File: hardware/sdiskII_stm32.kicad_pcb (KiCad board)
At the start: 2 copper layers, 67 x 55.5 mm, 8 parts, among them J2 APPLE_SDISKII, U2 MicroSD_SDIO, U8 DM-OLED096-636

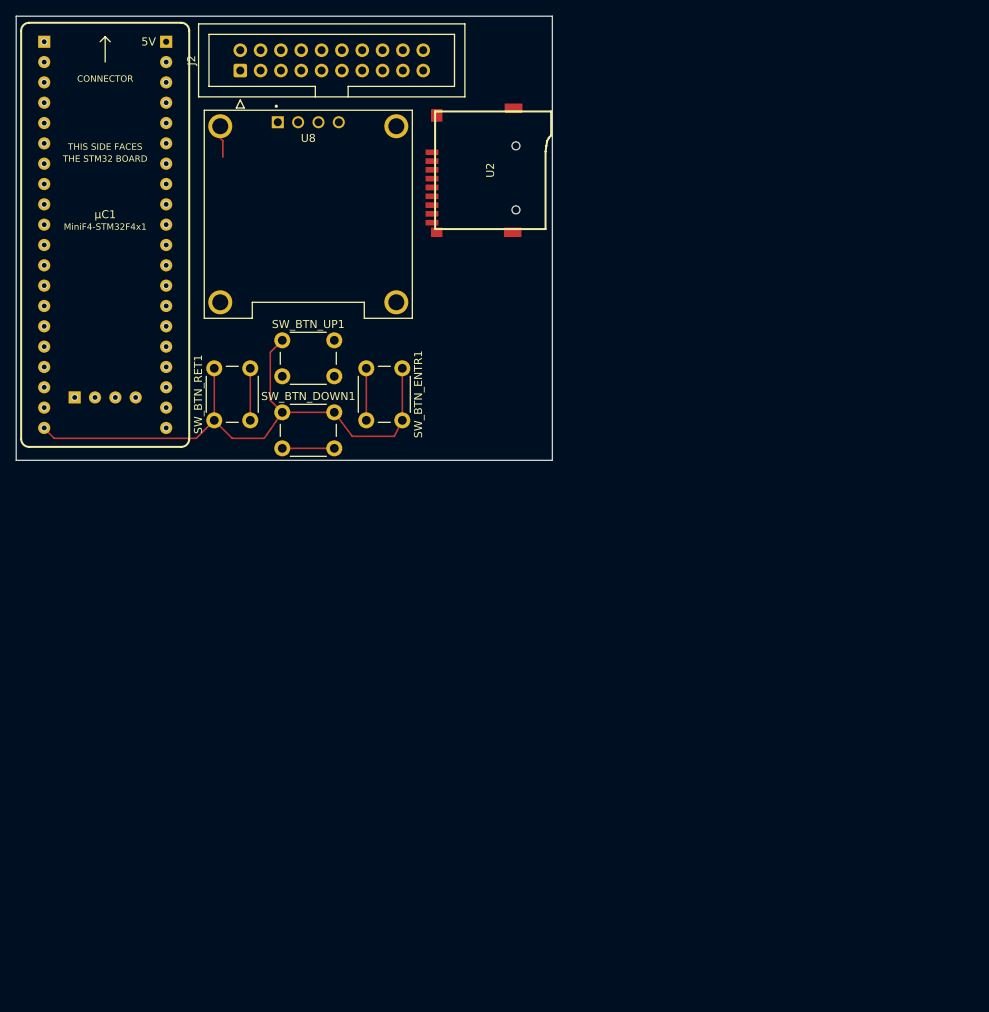
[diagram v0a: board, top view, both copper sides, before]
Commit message: new realease with gerber
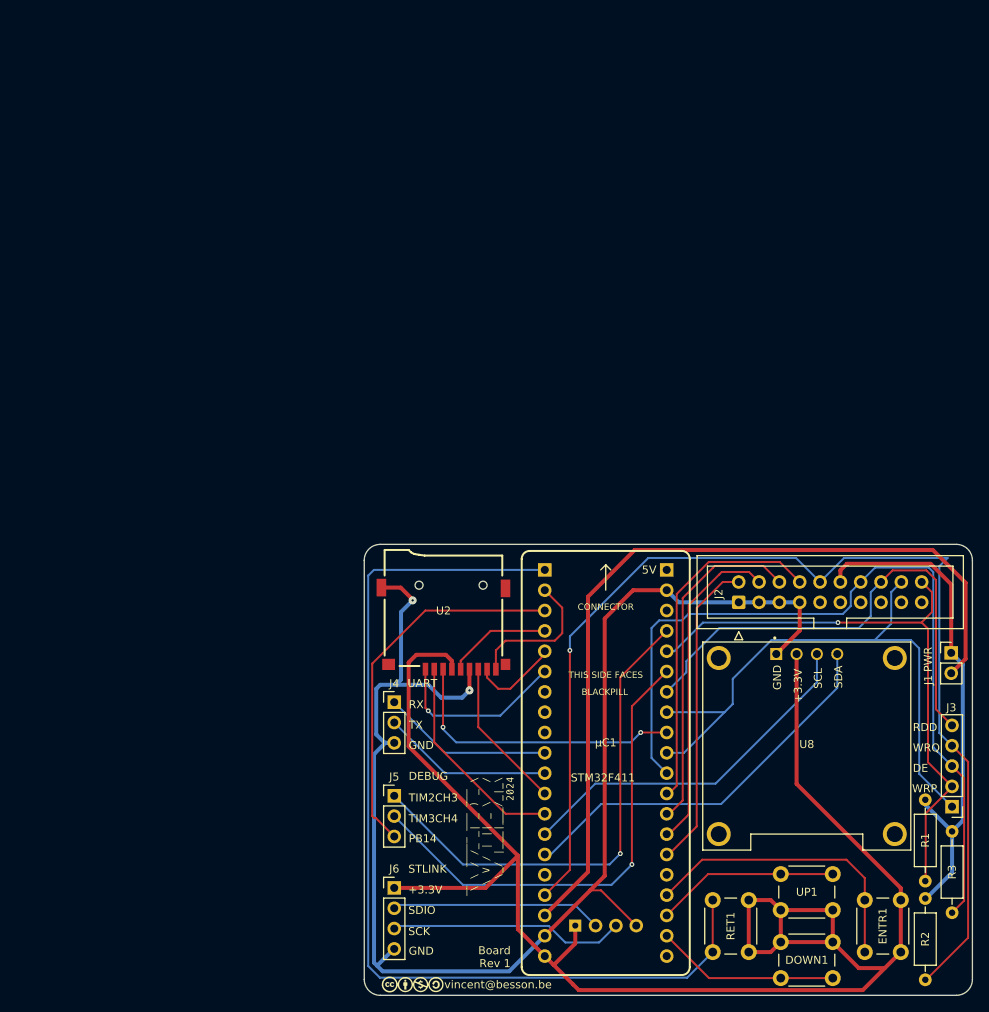
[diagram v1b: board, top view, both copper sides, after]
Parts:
- added  : LOGO, LOGO, F.Cu at (147.0, 121.7)
- added  : LOGO, LOGO, F.Cu at (138.6, 140.2)
- added J1: PWR, Connector_PinHeader_2.54mm:PinHeader_1x02_P2.54mm_Vertical, F.Cu at (204.8, 98.8)
- added J3: DBG, Connector_PinHeader_2.54mm:PinHeader_1x05_P2.54mm_Vertical, F.Cu at (204.9, 118.0)
- added J4: UART, Connector_PinHeader_2.54mm:PinHeader_1x03_P2.54mm_Vertical, F.Cu at (135.2, 105.0)
- added J5: TIM, Connector_PinHeader_2.54mm:PinHeader_1x03_P2.54mm_Vertical, F.Cu at (135.2, 116.7)
- added J6: STLINK, Connector_PinHeader_2.54mm:PinHeader_1x04_P2.54mm_Vertical, F.Cu at (135.2, 128.2)
- added R1: 1k, Resistor_THT:R_Axial_DIN0207_L6.3mm_D2.5mm_P10.16mm_Horizontal, F.Cu at (201.6, 127.3)
- added R2: 1k, Resistor_THT:R_Axial_DIN0207_L6.3mm_D2.5mm_P10.16mm_Horizontal, F.Cu at (201.6, 129.5)
- added R3: 1k, Resistor_THT:R_Axial_DIN0207_L6.3mm_D2.5mm_P10.16mm_Horizontal, F.Cu at (204.9, 121.1)
- U2: footprint sdisk_stm32:GCT-MEM2055-00-190-01-A -> sdisk_stm32:GCT-MEM2055-00-190-01-A_VIB
- μC1: footprint acheron_Hardware.pretty-master:Mini_F4X1_STM32 -> acheron_Hardware.pretty-master:Mini_F4X1_STM32_VIB
- moved UP1 99.0 mm to (190.0, 130.9), turned to 180 degrees
- moved U8 91.1 mm to (186.8, 110.5)
- moved ENTR1 91.1 mm to (198.5, 129.7)
- moved J2 91.1 mm to (178.3, 92.5)
- moved μC1 90.9 mm to (161.7, 112.6)
- moved DOWN1 90.9 mm to (183.5, 134.9)
- moved RET1 89.7 mm to (179.5, 129.7), turned to -90 degrees
- moved U2 63.2 mm to (141.4, 101.7), turned to 0 degrees
- renumbered SW_BTN_DOWN1 to DOWN1, SW_BTN_ENTR1 to ENTR1, SW_BTN_RET1 to RET1, SW_BTN_UP1 to UP1
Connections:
- J2 pad 14: DRIVE_ENABLE -> DEVICE_ENABLE
- U2 pad 10: (no net) -> GND
- U2 pad ~: (no net) -> GND
- μC1 pad 1: unconnected-(μC1-B12-Pad1) -> BTN_RET
- μC1 pad 18: unconnected-(μC1-5Vi-Pad18) -> PWR_IN
- μC1 pad 2: unconnected-(μC1-B13-Pad2) -> SD_EJECT
- μC1 pad 22: BTN_ENTR -> BTN_DOWN
- μC1 pad 24: BTN_DOWN -> BTN_ENTR
- μC1 pad 30: /DEVICE_ENABLE -> DEVICE_ENABLE
- μC1 pad 31: SP1_SCK -> WR_DATA
- μC1 pad 37: SD_EJECT -> TIM2_CH3
- μC1 pad 41: unconnected-(μC1-3.3V-Pad41) -> +3.3V
- μC1 pad 42: unconnected-(μC1-SDIO-Pad42) -> SDIO
- μC1 pad 43: unconnected-(μC1-SCK-Pad43) -> SCK
- μC1 pad 44: unconnected-(μC1-GND-Pad44) -> GND
- μC1 pad 7: TIM1_CH3 -> unconnected-(μC1-A10-Pad7)
- μC1 pad 8: BTN_RET -> unconnected-(μC1-A11-Pad8)
- μC1 pad 9: WR_DATA -> unconnected-(μC1-A12-Pad9)
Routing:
- net +3.3V: track 0.00 -> 208.6 mm
- net GND: track 0.00 -> 180.2 mm, vias 0 -> 2
- net WR_REQ: track 0.00 -> 144.3 mm, vias 0 -> 1
- net BTN_RET: track 0.00 -> 122.6 mm
- net PWR_IN: track 0.00 -> 105.4 mm
- net DEVICE_ENABLE: track 0.00 -> 103.3 mm
- net WR_DATA: track 0.00 -> 78.3 mm
- net WR_PROTECT: track 0.00 -> 74.7 mm, vias 0 -> 1
- net TIM2_CH3: track 0.00 -> 62.6 mm, vias 0 -> 1
- net RD_DATA: track 0.00 -> 62.5 mm
- net TIM3_CH4: track 0.00 -> 60.2 mm, vias 0 -> 1
- net VCC: track 3.92 -> 63.9 mm
- net I2C_SDA: track 0.00 -> 49.4 mm
- net DEBUG: track 0.00 -> 47.2 mm
- net I2C_SCL: track 0.00 -> 45.4 mm
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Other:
- board size 67 x 55.5 mm -> 76 x 56.3 mm
- board text added: "+3.3V"
- board text added: "Board Rev 1"
- board text added: "DE"
- board text added: "DEBUG"
- board text added: "GND"
- board text added: "PB14"
- board text added: "PWR"
- board text added: "RDD"
- board text added: "RX"
- board text added: "SCK"
- board text added: "SCL"
- board text added: "SDA"
- board text added: "SDIO"
- board text added: "STLINK"
- board text added: "STM32F411"
- board text added: "TIM2CH3"
- board text added: "TIM3CH4"
- board text added: "TX"
- board text added: "UART"
- board text added: "WRP"
- board text added: "WRQ"
- board text added: "vincent@besson.be"
